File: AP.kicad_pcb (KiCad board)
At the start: 2 copper layers, 71 x 54 mm, 21 parts, among them U1 74HC04, U2 74HC04

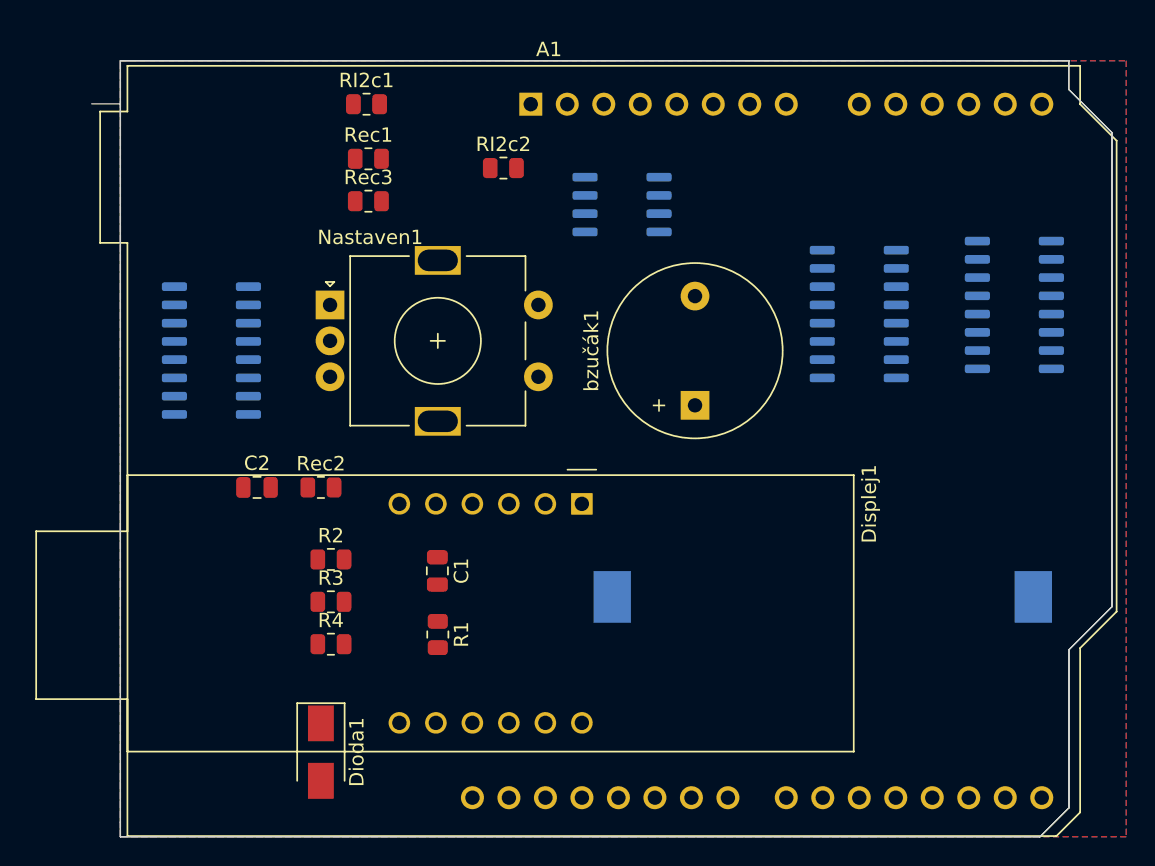
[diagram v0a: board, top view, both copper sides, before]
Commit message: 1
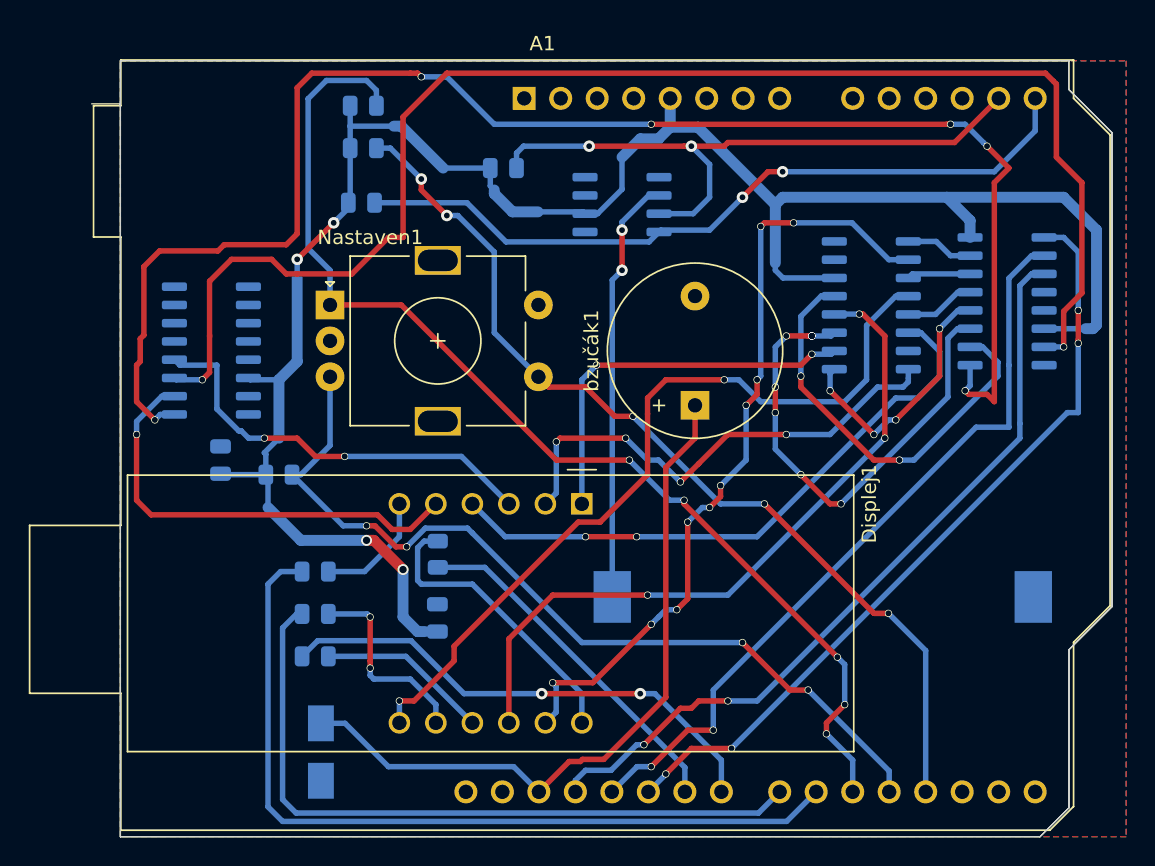
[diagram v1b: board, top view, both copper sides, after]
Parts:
- C1, C2, Dioda1, R1, R2, R3, R4, RI2c1, RI2c2, Rec1, Rec2, Rec3: moved to B.Cu
- moved RI2c1 6.87 mm to (150.8, 79.9)
- moved R2 6.83 mm to (147.6, 111.4)
- moved Rec3 6.65 mm to (150.9, 73.1)
- moved R1 5.59 mm to (156.1, 104.3), turned to 90 degrees
- moved R4 5.17 mm to (147.6, 105.5)
- moved C1 3.27 mm to (156.1, 108.8), turned to 90 degrees
- moved C2 3.17 mm to (141.0, 97.8), turned to 90 degrees
- moved Rec2 3.05 mm to (145.0, 98.8)
- moved R3 1.38 mm to (147.6, 108.5)
- moved U1 1.04 mm to (186.3, 87.0)
- moved Rec1 0.82 mm to (150.9, 76.1)
- moved A1 0.61 mm to (162.1, 72.6)
- moved Demultiplexor1 0.57 mm to (195.7, 86.7)
- turned Dioda1 to 90 degrees
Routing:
- net VCC: track 0.00 -> 140.5 mm, vias 0 -> 4
- net Y6: track 0.00 -> 108.3 mm, vias 0 -> 6
- net Y7: track 0.00 -> 101.0 mm, vias 0 -> 2
- net A: track 0.00 -> 78.1 mm, vias 0 -> 5
- net S1: track 0.00 -> 66.3 mm, vias 0 -> 5
- net B: track 0.00 -> 60.9 mm, vias 0 -> 4
- net GNDs6: track 0.00 -> 57.7 mm
- net Net-(Displej1-Pad7): track 0.00 -> 55.8 mm, vias 0 -> 2
- net A0: track 0.00 -> 54.8 mm, vias 0 -> 4
- net Net-(Displej1-Pad11): track 0.00 -> 54.8 mm, vias 0 -> 10
- net A2: track 0.00 -> 54.2 mm, vias 0 -> 2
- net A1: track 0.00 -> 53.2 mm, vias 0 -> 2
- net SCL: track 0.00 -> 52.6 mm, vias 0 -> 2
- net Buz: track 0.00 -> 49.9 mm
- net GNDs8: track 0.00 -> 49.3 mm
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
